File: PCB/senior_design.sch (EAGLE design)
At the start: 23 parts, among them IC1 INA118P, IC2 TLC272P

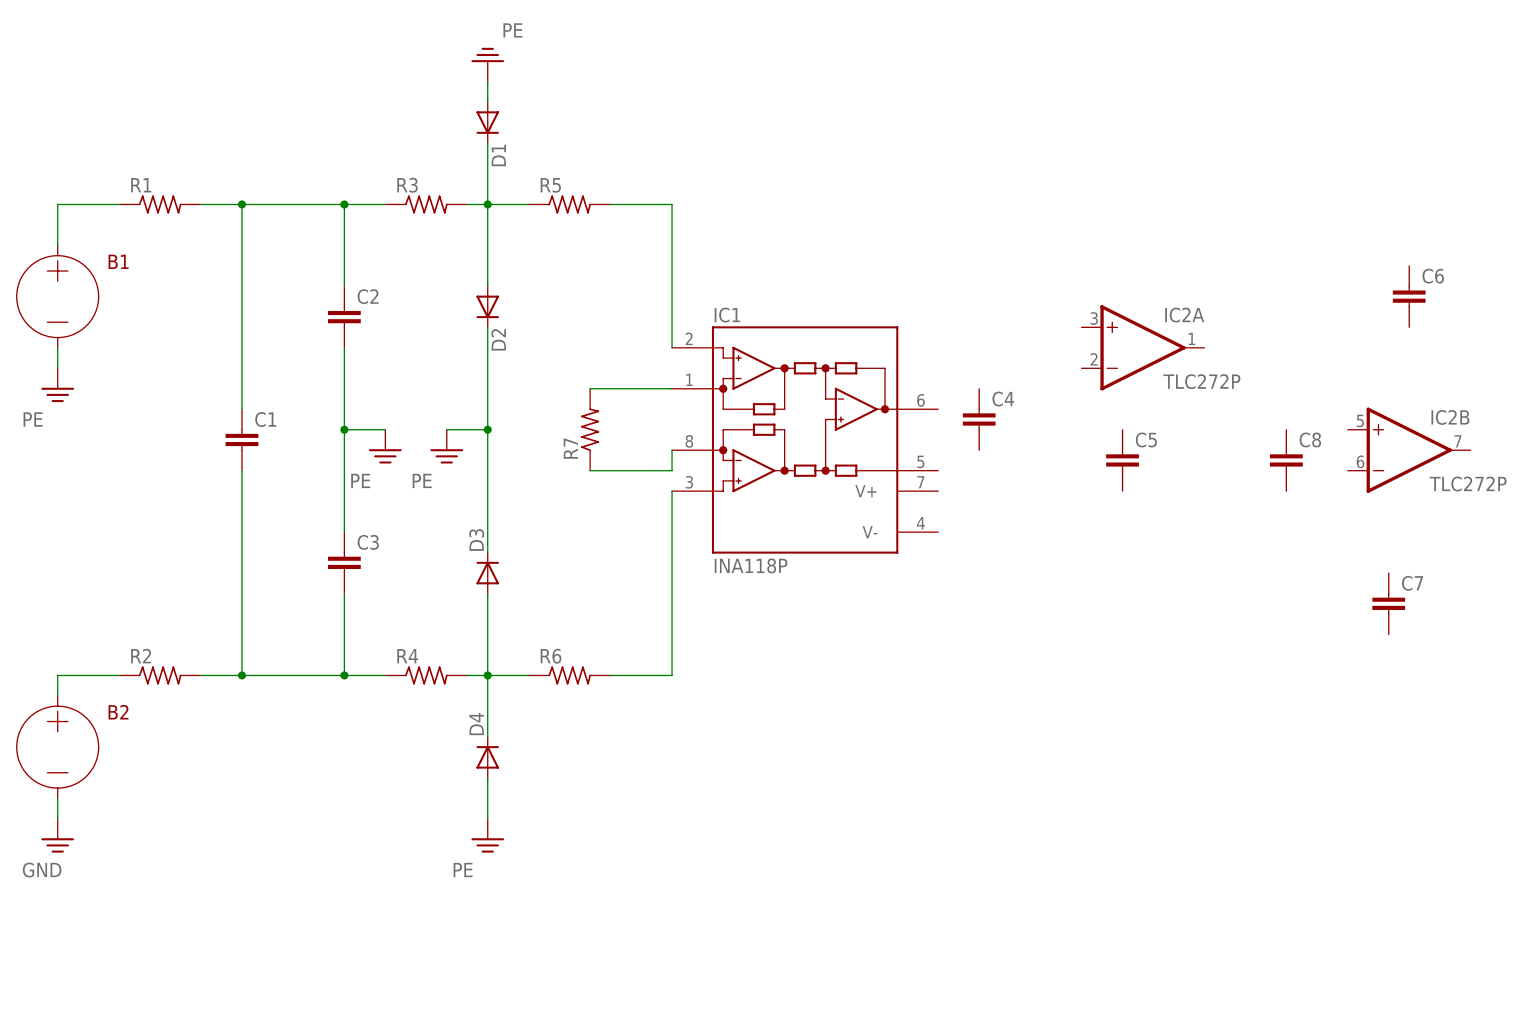
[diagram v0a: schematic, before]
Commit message: Updated schematics and pcb
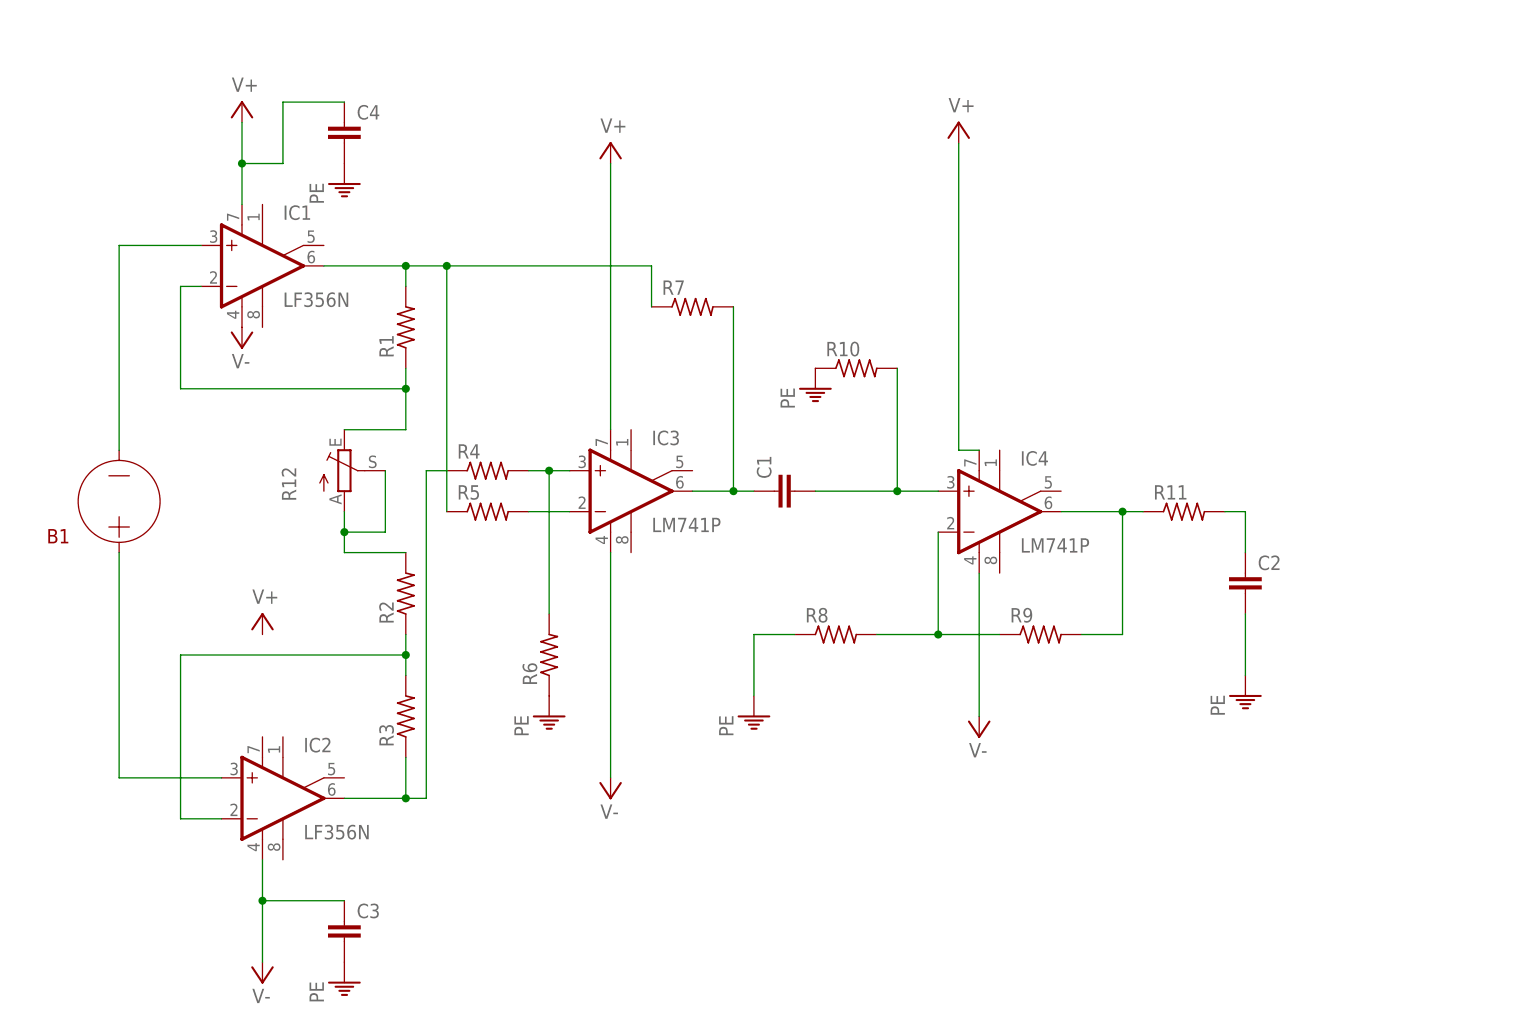
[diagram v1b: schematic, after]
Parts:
- removed B2: (no value), ngspice-simulation:NONLIN_ASRC
- removed C5, C6, C7, C8: (no value), capacitor-wima:C2,5-3
- removed D1, D2, D3, D4: 1N4148DO35-7, diode:1N4148DO35-7
- added IC3, IC4: LM741P, linear:LM741P
- added R10, R11, R8, R9: (no value), rcl:R-US_0204/7
- added R12: (no value), pot:TRIM_EU-B25X
- IC1: value INA118P -> LF356N; device burr-brown:INA118P -> linear:LF356N
- IC2: value TLC272P -> LF356N; device linear:TLC272P -> linear:LF356N
- R1, R2, R3, R4, R5, R6, R7: device rcl:R-US_0204/2V -> rcl:R-US_0204/7
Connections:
- removed net N$9: IC1.RG, R7.2
- new net N$11: C1.1, IC3.OUT, R7.2
- new net N$12: IC4.-IN, R8.2, R9.1
- new net N$13: IC4.OUT, R11.1, R9.2
- new net N$15: C2.1, R11.2
- new net N$17: R12.A, R12.S, R2.2
- new net V+: C4.1, IC1.V+, IC3.V+, IC4.V+
- new net V-: C3.1, IC1.V-, IC2.V-, IC3.V-, IC4.V-
- net N$1: now also B1.-, IC1.+IN; no longer B1.+, R1.1
- net N$10: now also C1.2, IC4.+IN, R10.2; no longer IC1.RG@1, R7.1
- net N$2: now also B1.+, IC2.+IN; no longer B2.+, R2.1
- net N$3: now also IC1.OUT, R5.1, R7.1; no longer C1.1, C2.1, R3.1
- net N$4: now also IC1.-IN, R1.1, R12.E; no longer C1.2, C3.2, R2.2, R4.1
- net N$5: now also IC2.OUT, R3.1, R4.1; no longer D1.C, D2.A, R3.2, R5.1
- net N$6: now also IC2.-IN, R2.1, R3.2; no longer D3.A, D4.C, R4.2, R6.1
- net N$7: now also IC3.+IN, R4.2, R6.2; no longer IC1.-IN, R5.2
- net N$8: now also IC3.-IN, R5.2; no longer IC1.+IN, R6.2
- net PE: now also C3.2, C4.2, R10.1, R6.1, R8.1; no longer B1.-, B2.-, C3.1, D1.A, D2.C, D3.C, D4.A
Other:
- moved on the sheet: B1, C1, C2, C3, C4, R1, R2, R3, R4, R5, R6, R7
